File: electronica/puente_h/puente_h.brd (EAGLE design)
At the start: 80.2 x 123.2 mm, 40 parts, among them IC1 7805, IC2 7812, IC3 7404LP, IC4 7408LP, IC5 ADUM1400, Q1 IRF2804, Q2 IRF2804, Q5 IRF2804, Q6 IRF2804, U1 IR2110LP

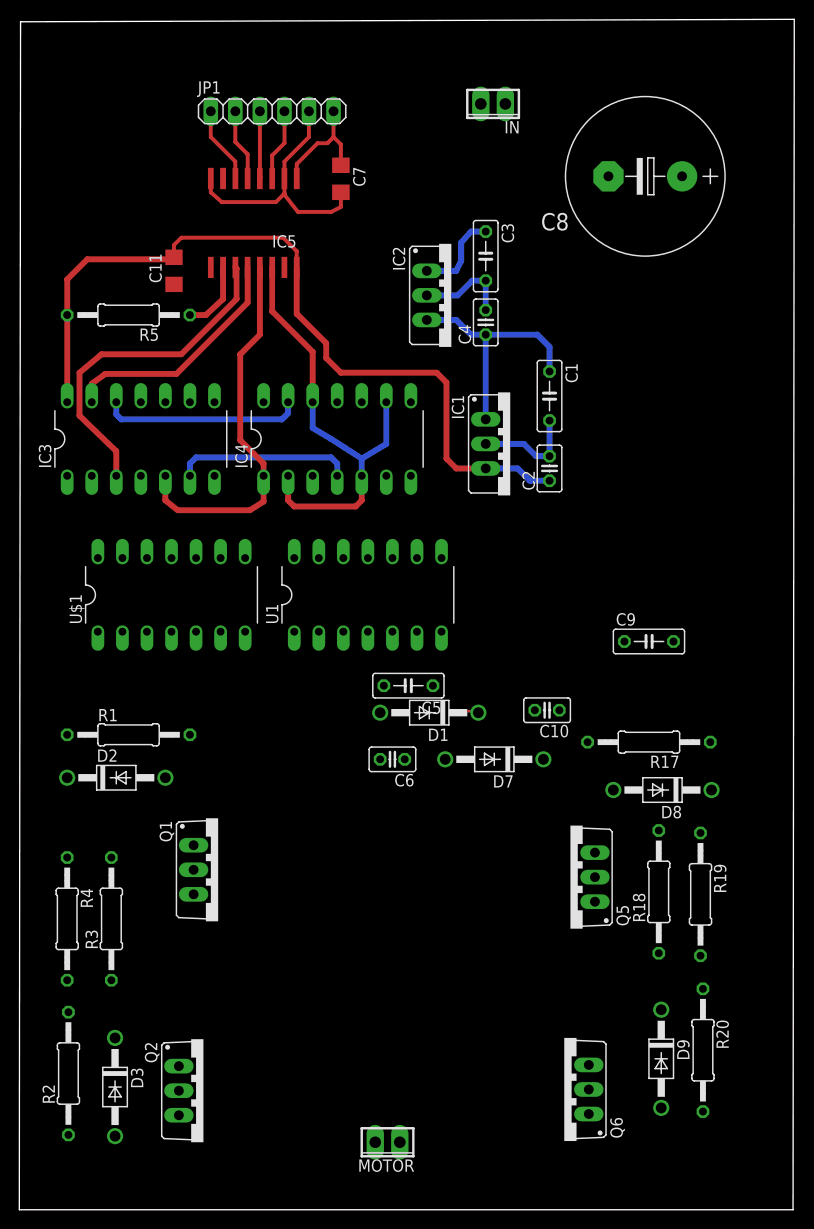
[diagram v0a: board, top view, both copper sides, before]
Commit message: mejores posiciones
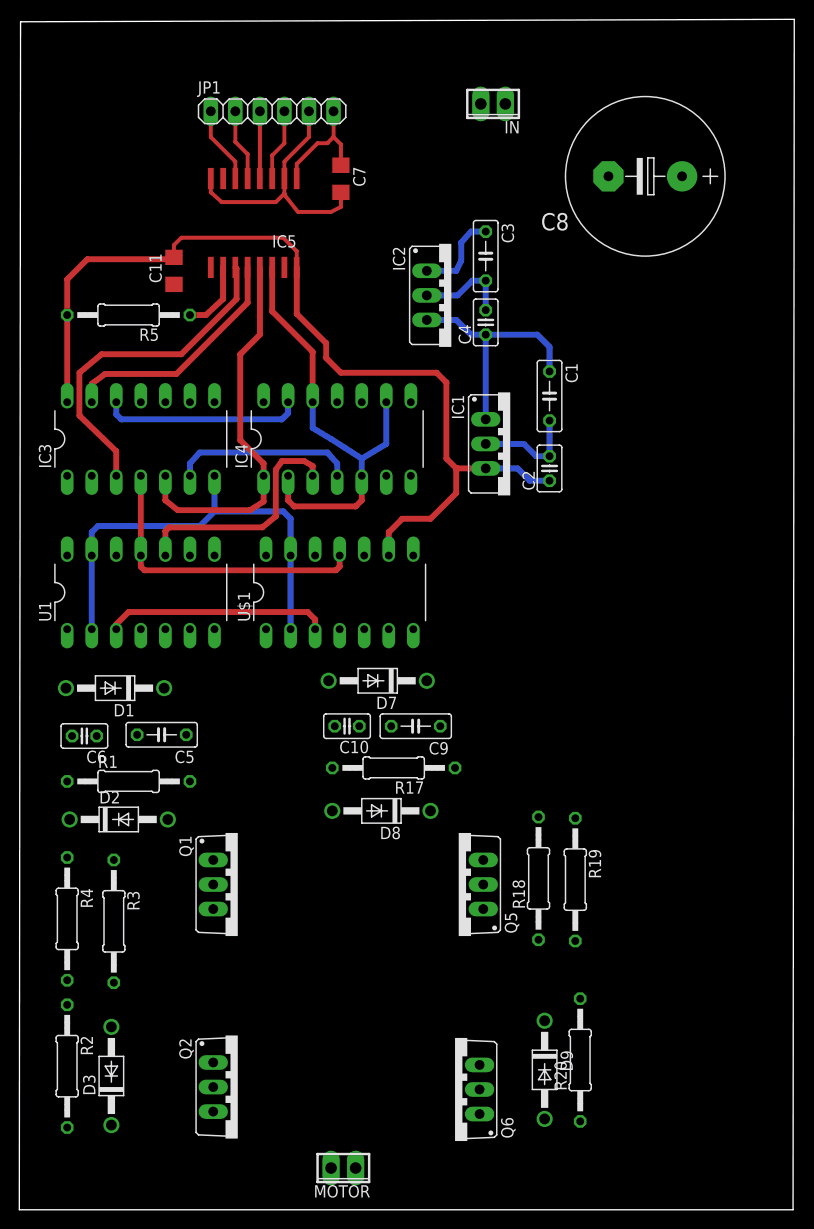
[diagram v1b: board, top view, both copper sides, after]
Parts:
- moved D1 32.6 mm to (11.3, 58.0)
- moved C6 32.0 mm to (6.86, 53.1)
- moved D8 29.2 mm to (38.9, 45.3)
- moved R17 26.6 mm to (38.9, 49.8)
- moved C5 26.0 mm to (14.9, 53.2)
- moved C9 25.7 mm to (41.1, 54.1), turned to 180 degrees
- moved U1 23.5 mm to (11.4, 67.9)
- moved C10 20.8 mm to (34.0, 54.1)
- moved U$1 17.4 mm to (32.0, 67.9)
- moved D7 14.5 mm to (38.5, 58.8)
- moved R19 13.0 mm to (57.7, 38.2)
- moved R20 12.7 mm to (58.2, 19.6), turned to 90 degrees
- moved R18 12.5 mm to (53.8, 38.4)
- moved D9 12.1 mm to (54.5, 19.8)
- moved Q5 11.6 mm to (45.6, 37.7)
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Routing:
- net GND: track 20.6 -> 67.6 mm
- net SD: track 0.00 -> 31.4 mm
- net N$11: track 0.00 -> 24.8 mm
- net +12V: track 25.2 -> 48.1 mm
- net +5V: track 84.9 -> 98.6 mm
- net N$1: track 2.37 -> 0.00 mm
- net N$7: track 1.46 -> 0.23 mm
- net N$36: track 0.55 -> 0.00 mm
- net N$10: track 18.3 -> 18.8 mm

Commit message: ruteo mejorado
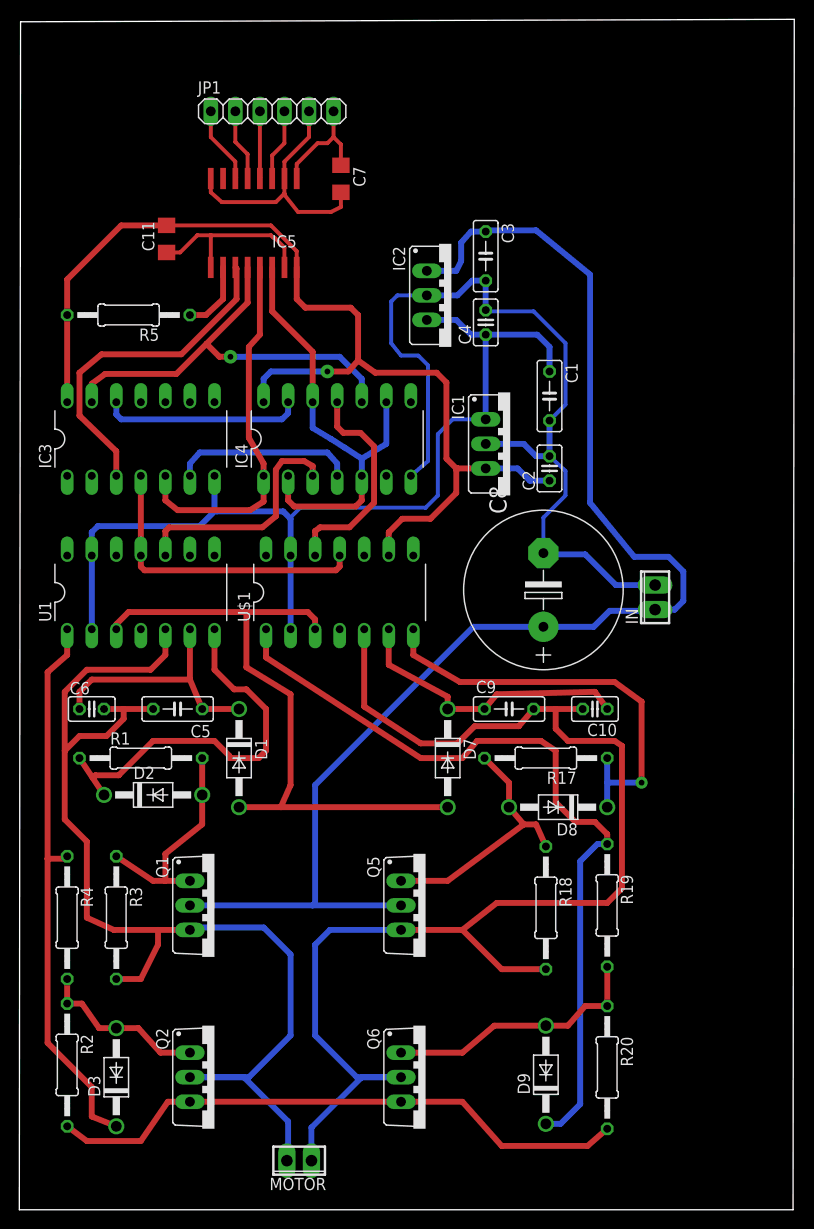
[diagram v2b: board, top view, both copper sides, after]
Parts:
- moved IN 53.7 mm to (65.9, 67.4), turned to 90 degrees
- moved C8 44.1 mm to (54.4, 68.2), turned to 90 degrees
- moved C10 25.7 mm to (59.7, 55.9)
- moved D8 18.3 mm to (57.1, 45.7)
- moved R17 15.8 mm to (54.6, 50.8)
- moved D1 13.0 mm to (22.9, 52.1), turned to 270 degrees
- moved C9 9.81 mm to (50.8, 55.9), turned to 0 degrees
- moved D7 9.00 mm to (44.5, 52.1), turned to 270 degrees
- moved MOTOR 4.64 mm to (29.1, 9.14)
- moved D2 4.37 mm to (12.7, 47.0)
- moved R19 4.24 mm to (61.0, 35.6)
- moved Q5 4.05 mm to (42.2, 35.6), turned to 270 degrees
- moved C11 3.39 mm to (15.4, 104.5)
- moved Q6 3.30 mm to (42.2, 17.8), turned to 270 degrees
- moved Q1 3.24 mm to (20.3, 35.6)
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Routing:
- net GND: track 67.6 -> 216.1 mm
- net N$31: track 0.00 -> 136.8 mm
- net VIN: track 9.14 -> 141.6 mm
- net N$3: track 0.00 -> 119.9 mm
- net N$35: track 0.00 -> 83.2 mm
- net +12V: track 48.1 -> 120.8 mm
- net N$6: track 0.00 -> 58.1 mm
- net N$32: track 0.00 -> 44.7 mm, vias 0 -> 1
- net N$2: track 0.00 -> 40.8 mm
- net N$30: track 0.00 -> 30.0 mm
- net N$36: track 0.00 -> 27.3 mm
- net N$33: track 0.00 -> 26.9 mm
- net N$1: track 0.00 -> 26.1 mm
- net N$4: track 0.00 -> 22.9 mm
- net N$19: track 0.00 -> 22.8 mm
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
